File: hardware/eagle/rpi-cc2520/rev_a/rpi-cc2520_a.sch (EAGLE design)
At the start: 18 parts, among them J1 PINHD-2X12/SMD, J2 PINHD-2X12/SMD, U1 CC2520

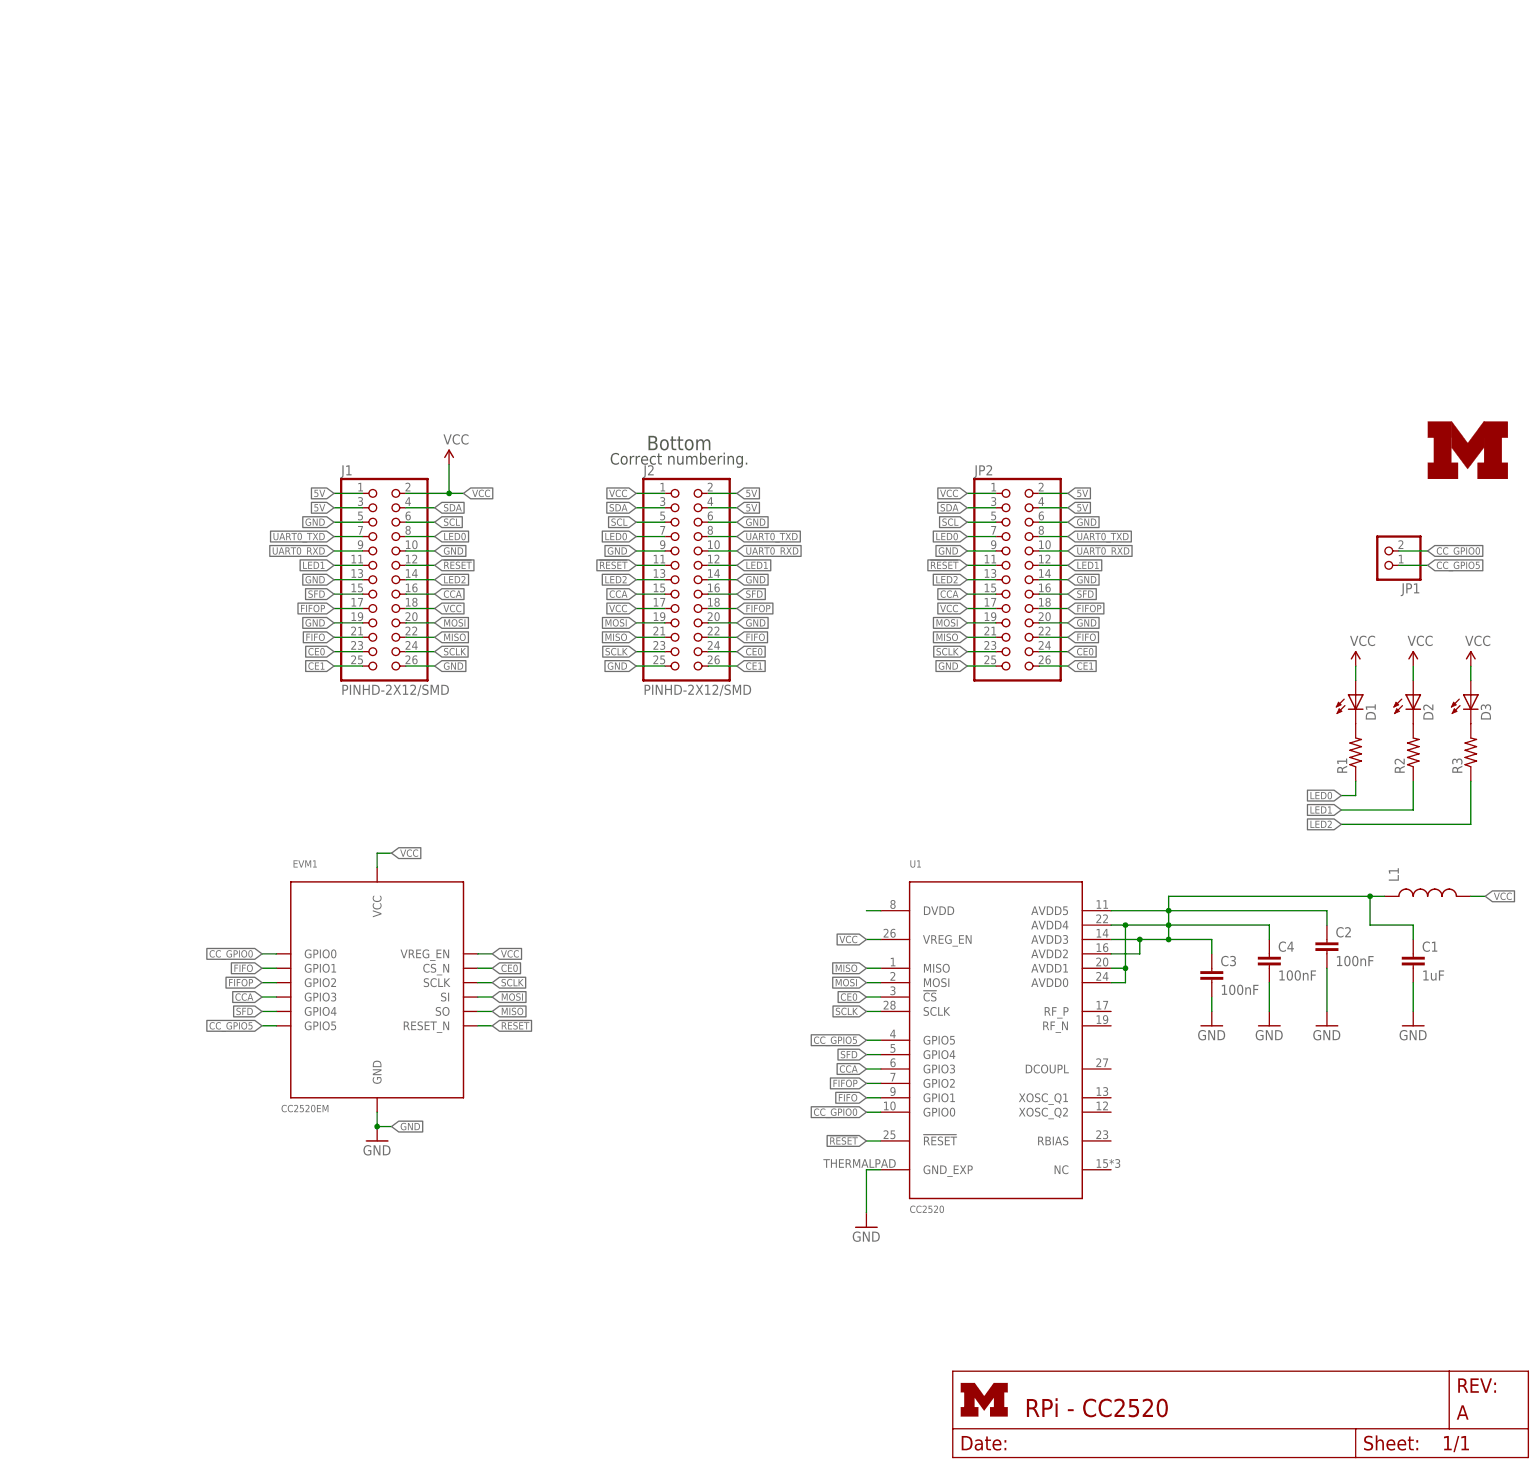
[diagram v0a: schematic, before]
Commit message: working on rf path
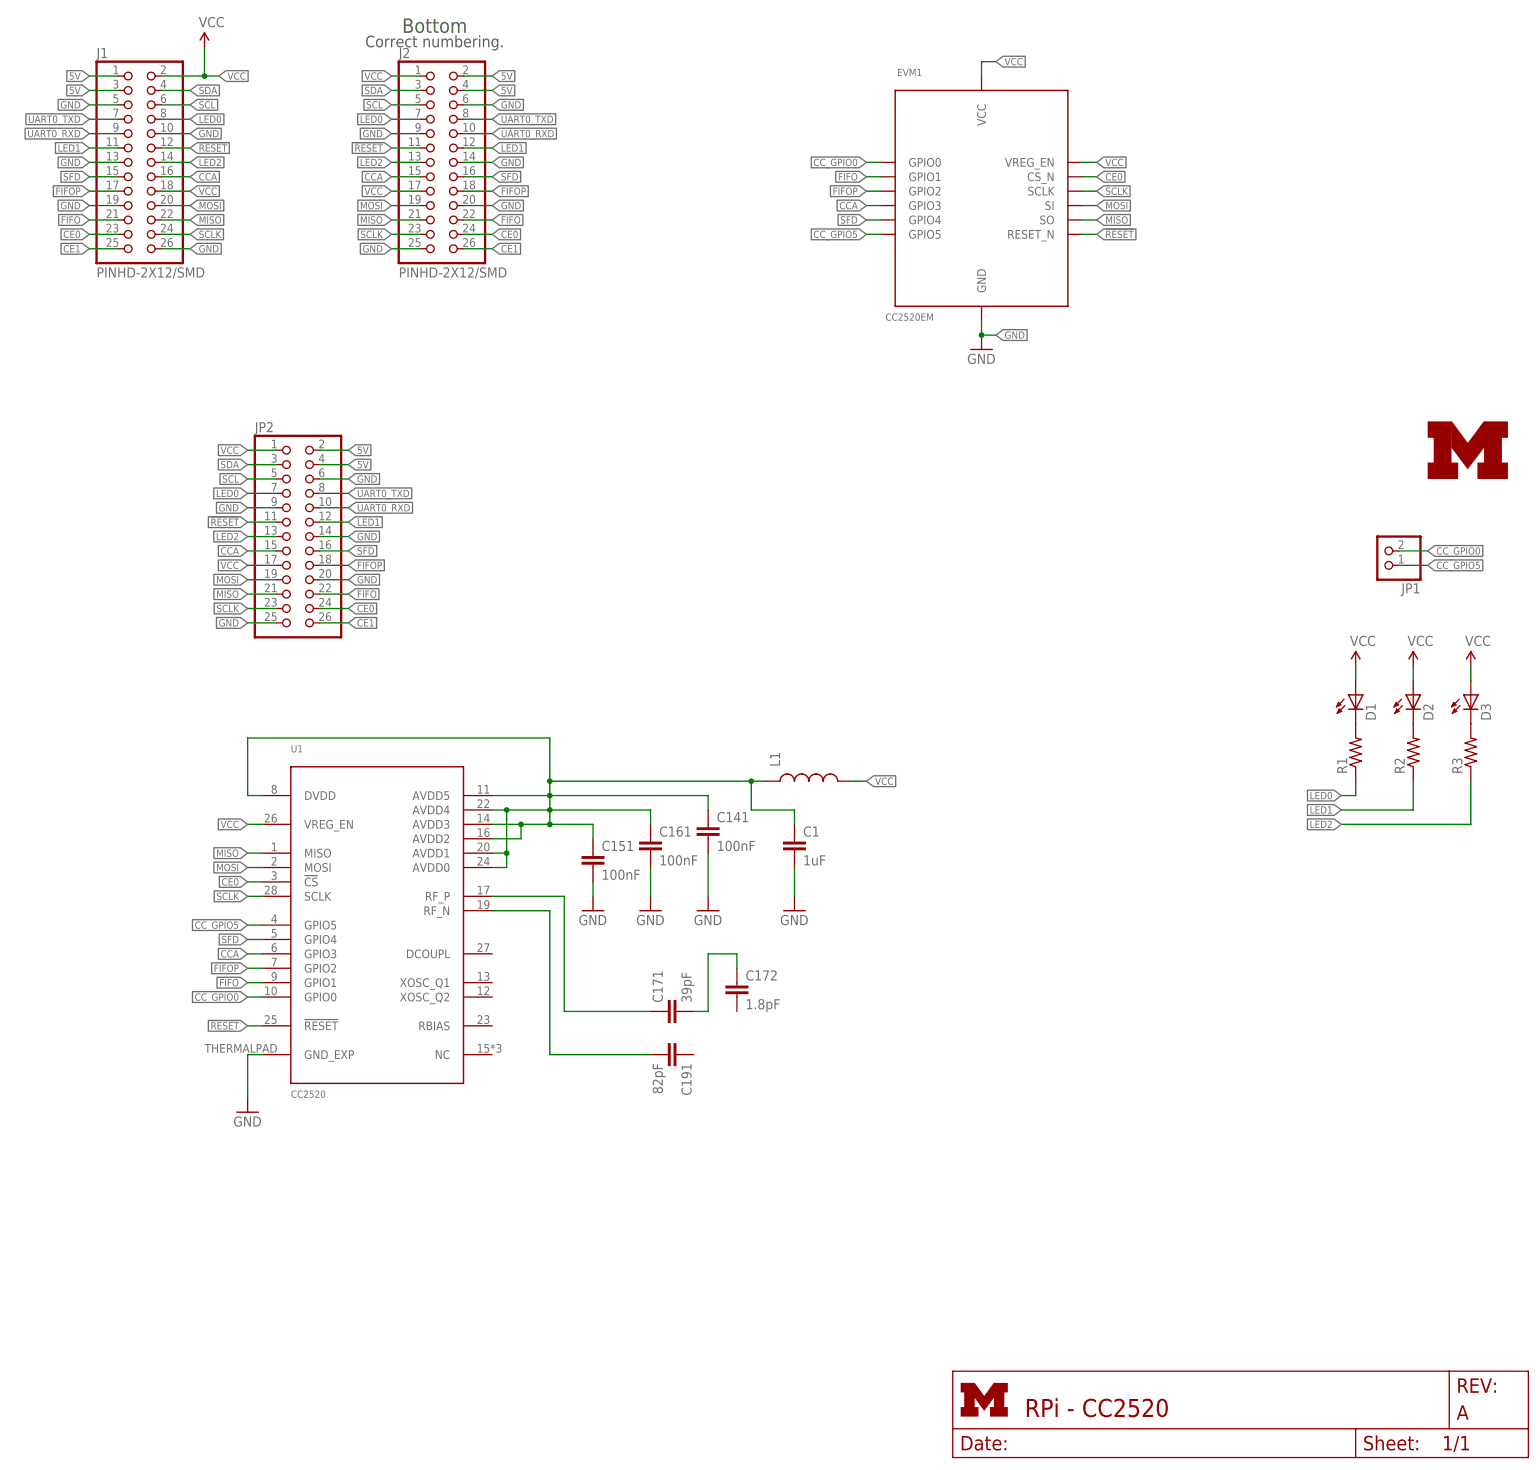
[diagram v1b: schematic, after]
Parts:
- removed C2, C3, C4: 100nF, rcl:C-EUC0402
- added C141, C151, C161: 100nF, rcl:C-EUC0402
- added C171: 39pF, rcl:C-EUC0402
- added C172: 1.8pF, rcl:C-EUC0402
- added C191: 82pF, rcl:C-EUC0402
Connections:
- new net N$6: C191.2, U1.RF_N
- new net N$7: C171.2, C172.1
- net GND: now also C141.2, C151.2, C161.2; no longer C2.2, C3.2, C4.2
- net N$4: now also C171.1, U1.RF_P; no longer C1.1, C2.1, C3.1, C4.1, L1.1, U1.AVDD0, U1.AVDD1, U1.AVDD2, U1.AVDD3, U1.AVDD4, U1.AVDD5
- net N$5: now also C1.1, C141.1, C151.1, C161.1, L1.1, U1.AVDD0, U1.AVDD1, U1.AVDD2, U1.AVDD3, U1.AVDD4, U1.AVDD5
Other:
- moved on the sheet: C1, EVM1, J1, J2, JP2, L1, U1
